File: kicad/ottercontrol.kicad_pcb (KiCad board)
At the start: 2 copper layers, 97.8 x 52.1 mm, 114 parts, among them IC1 MAX485, IC2 USBLC6-4, IC3 USBLC6-2SC6, J1 USB_B_Micro, P1 Conn_01x02, Q1 Q_PMOS_GSD, Q2 IRF3205, Q3 IRF3205, Q4 IRF3205, Q5 IRF3205, Q6 IRF3205, Q7 IRF3205, U1 STM32F303CBT6, U2 MAX3051, U3 MIC4605, U4 MIC4605, U5 MIC4605, U6 XL7015, U7 ACT4088, U8 MIC5504-3.3YM5, X1 programmer, X2 Conn_01x08, X3 Conn_01x05, Y1 16MHz

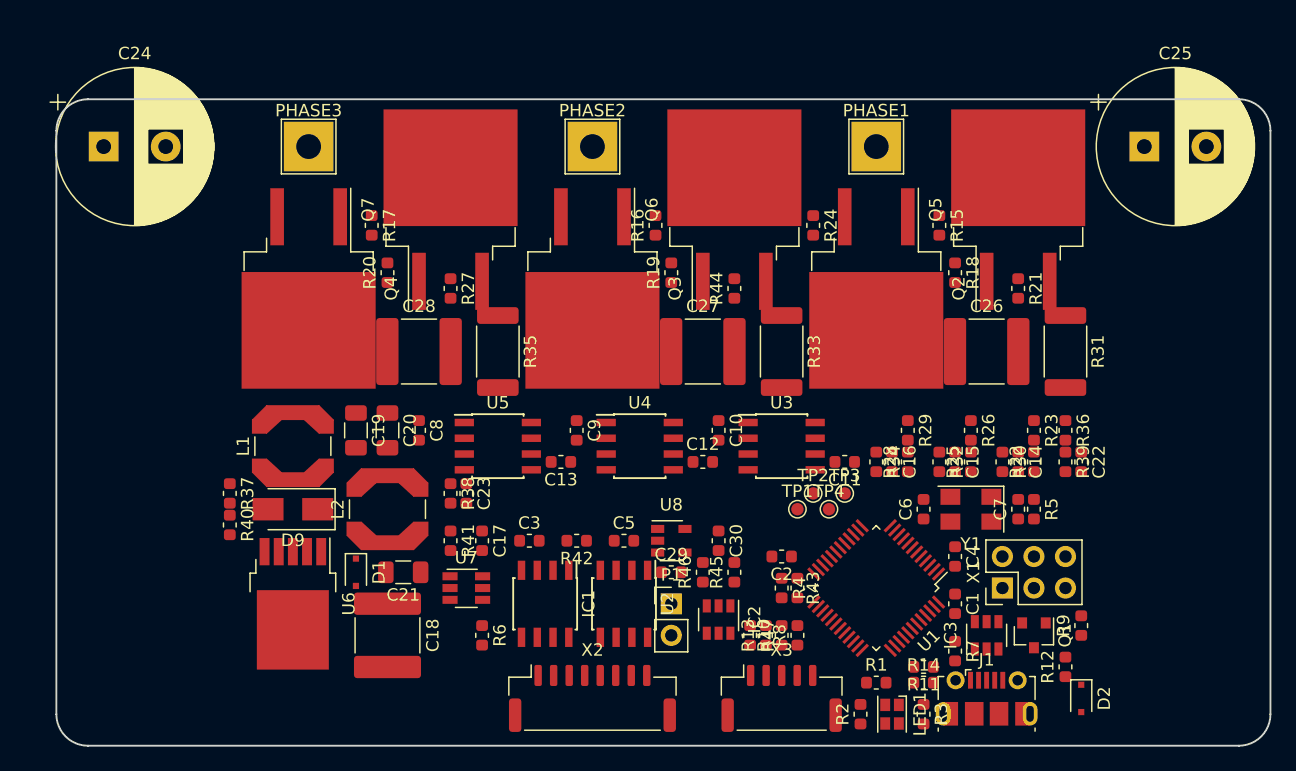
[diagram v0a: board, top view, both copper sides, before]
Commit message: placed and routed; preliminary finished
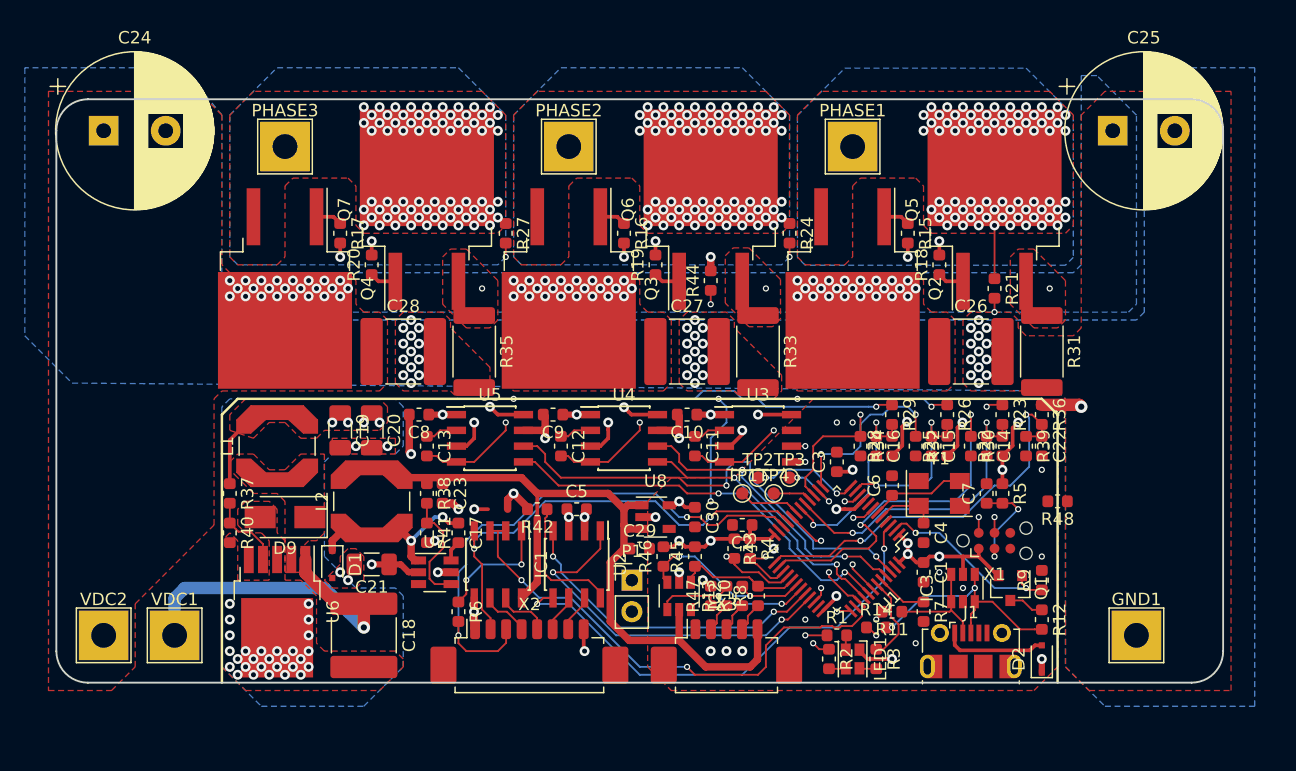
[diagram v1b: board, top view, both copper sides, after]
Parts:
- added GND1: Conn_01x01, TestPoint:TestPoint_THTPad_4.0x4.0mm_Drill2.0mm, F.Cu at (140.3, 80.0)
- added R48: 0, Resistor_SMD:R_0603_1608Metric, F.Cu at (134.0, 69.2)
- added VDC1: Conn_01x01, TestPoint:TestPoint_THTPad_4.0x4.0mm_Drill2.0mm, F.Cu at (62.9, 80.0)
- added VDC2: Conn_01x01, TestPoint:TestPoint_THTPad_4.0x4.0mm_Drill2.0mm, F.Cu at (57.1, 80.0)
- X1: footprint Connector_PinHeader_2.54mm:PinHeader_2x03_P2.54mm_Vertical -> Connector:Tag-Connect_TC2030-IDC-NL_2x03_P1.27mm_Vertical
- X2: footprint Connector_JST:JST_GH_SM08B-GHS-TB_1x08-1MP_P1.25mm_Horizontal -> Connector_Molex:Molex_PicoBlade_53261-0871_1x08-1MP_P1.25mm_Horizontal
- X3: footprint Connector_JST:JST_GH_SM05B-GHS-TB_1x05-1MP_P1.25mm_Horizontal -> Connector_Molex:Molex_PicoBlade_53261-0571_1x05-1MP_P1.25mm_Horizontal
- moved C3 25.6 mm to (116.2, 66.0), turned to 90 degrees
- moved C11 12.1 mm to (104.8, 64.8), turned to 270 degrees
- moved C12 11.5 mm to (94.0, 64.8), turned to 270 degrees
- moved C13 10.9 mm to (83.2, 64.8), turned to 270 degrees
- moved R27 6.29 mm to (89.5, 47.6)
- moved R43 5.99 mm to (108.0, 73.0)
- moved X2 5.99 mm to (91.4, 81.9)
- moved R14 5.85 mm to (119.4, 79.4)
- moved R3 5.85 mm to (119.4, 81.9)
- moved X3 5.46 mm to (107.3, 81.9)
- moved LED1 5.46 mm to (117.5, 81.9)
- moved R2 5.12 mm to (115.6, 81.9), turned to 270 degrees
- moved R11 5.12 mm to (120.7, 78.1)
- moved U2 4.96 mm to (95.2, 74.3)
- moved IC1 4.96 mm to (88.9, 74.3)
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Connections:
- net Net-(R15-Pad2) renamed /Phase Driver 1/HO
- net Net-(R16-Pad2) renamed /Phase Driver 2/HO
- net Net-(R17-Pad2) renamed /Phase Driver 3/HO
- net Net-(R18-Pad2) renamed /Phase Driver 1/LO
- net Net-(R19-Pad2) renamed /Phase Driver 2/LO
- net Net-(R20-Pad2) renamed /Phase Driver 3/LO
- C5 pad 1: +5V -> +3V3
- IC1 pad 4: /RS458_TX -> /RS485_TX
- IC2 pad 5: +3V3 -> +5V
- IC3 pad 4: Net-(IC3-Pad4) -> Net-(IC3-Pad3)
- IC3 pad 6: Net-(IC3-Pad6) -> Net-(IC3-Pad1)
- R11 pad 1: Net-(IC3-Pad6) -> Net-(IC3-Pad1)
- R12 pad 2: Net-(IC3-Pad4) -> Net-(IC3-Pad3)
- R14 pad 2: Net-(IC3-Pad4) -> Net-(IC3-Pad3)
- U1 pad 21: /RS458_TX -> /RS485_TX
- U2 pad 3: +5V -> +3V3
- X3 pad 5: +3V3 -> +5V
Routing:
- net +12V: track 0.00 -> 67.1 mm, vias 0 -> 9
- net +5V: track 0.00 -> 66.8 mm
- net +3V3: track 0.00 -> 66.0 mm, vias 0 -> 18
- net /VSENS3: track 0.00 -> 52.0 mm, vias 0 -> 2
- net GND: track 0.00 -> 48.3 mm, vias 0 -> 26
- net /RS485_RX: track 0.00 -> 43.9 mm, vias 0 -> 2
- net Net-(Q7-Pad3): track 0.00 -> 41.3 mm, vias 0 -> 3
- net /RS485_DE: track 0.00 -> 40.7 mm, vias 0 -> 2
- net /Phase Driver 1/PHASE: track 0.00 -> 40.1 mm, vias 0 -> 74
- net /CAN_EN: track 0.00 -> 39.5 mm, vias 0 -> 2
- net /CAN_TX: track 0.00 -> 39.3 mm, vias 0 -> 3
- net /VSENS1: track 0.00 -> 39.1 mm, vias 0 -> 3
- net /PWML3: track 0.00 -> 37.6 mm, vias 0 -> 2
- net +VDC: track 0.00 -> 37.6 mm, vias 0 -> 74
- net /VSENS2: track 0.00 -> 37.5 mm, vias 0 -> 3
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- added copper zone on F.Cu, net +12V
- added copper zone on In1.Cu, net +12V
- added copper zone on In1.Cu, net +3V3
- added copper zone on B.Cu, net +VDC
- added copper zone on F.Cu, net +VDC
- added copper zone on In1.Cu, net +VDC
- added copper zone on B.Cu, net /Phase Driver 1/PHASE
- added copper zone on F.Cu, net /Phase Driver 1/PHASE
- added copper zone on B.Cu, net /Phase Driver 2/PHASE
- added copper zone on F.Cu, net /Phase Driver 2/PHASE
- added copper zone on B.Cu, net /Phase Driver 3/PHASE
- added copper zone on F.Cu, net /Phase Driver 3/PHASE
- added copper zone on F.Cu, net GND
- added copper zone on In2.Cu, net GND
- added copper zone on B.Cu, net GNDPWR
- added copper zone on F.Cu, net GNDPWR
- added copper zone on In2.Cu, net GNDPWR
- added copper zone on F.Cu, net Net-(D9-Pad1)
- added copper zone on F.Cu, net Net-(Q5-Pad3)
- added copper zone on F.Cu, net Net-(Q6-Pad3)
- added copper zone on F.Cu, net Net-(Q7-Pad3)
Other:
- board size 97.8 x 52.1 mm -> 94 x 47 mm
- copper layers 2 -> 4
- net class 0.3mm added: clearance 0.2, trace_width 0.3, via_dia 0.8, via_drill 0.4
- net class 0.5mm added: clearance 0.2, trace_width 0.5, via_dia 0.8, via_drill 0.4
- net class 0.6mm added: clearance 0.2, trace_width 0.6, via_dia 0.8, via_drill 0.4
- net class 1.0mm added: clearance 0.2, trace_width 1, via_dia 1, via_drill 0.5
- net class Default: trace_width 0.25 -> 0.15; via_dia 0.8 -> 0.5; via_drill 0.4 -> 0.3
- net class High Power added: clearance 0.2, trace_width 0.8, via_dia 0.8, via_drill 0.4
- rule trace_min: 0.2 -> 0.15
- rule via_min_drill: 0.3 -> 0.25
- rule via_min_size: 0.4 -> 0.5
